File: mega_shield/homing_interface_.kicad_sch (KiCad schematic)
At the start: 15 parts, among them J8 T4040014031-000, J9 T4040014031-000, U14 4N35, U15 4N35

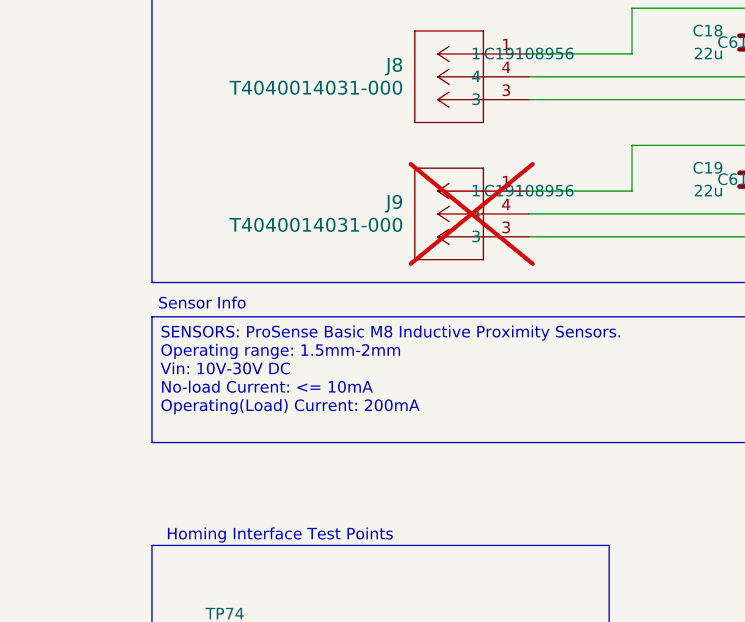
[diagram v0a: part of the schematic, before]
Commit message: replicated layout of homing interfaces. Placed the homing interface into PCB.
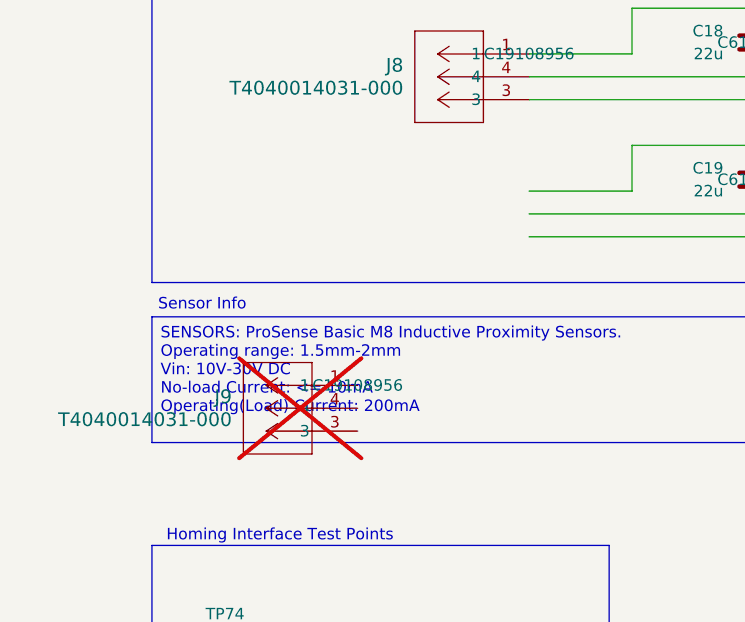
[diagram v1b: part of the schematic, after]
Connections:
- net +24V_IN: no longer J9.1
- net LIM_MAX_IN: no longer J9.3
- net at C19.2: no longer J9.4
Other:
- moved on the sheet: J9
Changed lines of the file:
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@@
 	(symbol
 		(lib_id "M8P3:T4040014031-000")
-		(at 67.31 62.23 0)
+		(at 48.26 83.82 0)
 		(mirror y)
 		(unit 1)
@@
 		(fields_autoplaced yes)
 		(property "Reference" "J9"
-			(at 53.34 63.4999 0)
+			(at 34.29 85.0899 0)
 			(effects
 				(font
@@
 		)
 		(property "Value" "T4040014031-000"
-			(at 53.34 66.0399 0)
+			(at 34.29 87.6299 0)
 			(effects
 				(font
@@
 		)
 		(property "Footprint" "footprints:CONN3_T4040014031-000_TEC"
-			(at 67.31 62.23 0)
+			(at 48.26 83.82 0)
 			(effects
 				(font
@@
 		)
 		(property "Datasheet" "T4040014031-000"
-			(at 67.31 62.23 0)
+			(at 48.26 83.82 0)
 			(effects
 				(font
@@
 		)
 		(property "Description" ""
-			(at 67.31 62.23 0)
+			(at 48.26 83.82 0)
 			(effects
 				(font
@@
 		)
 		(property "Purpose" ""
-			(at 67.31 62.23 0)
+			(at 48.26 83.82 0)
 			(effects
 				(font
@@
 		)
 		(property "jlcpcb" "C19108956"
-			(at 67.31 62.23 0)
+			(at 48.26 83.82 0)
 			(effects
 				(font

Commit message: fixed issue with shcematic connector having moved in homing interface sheet.
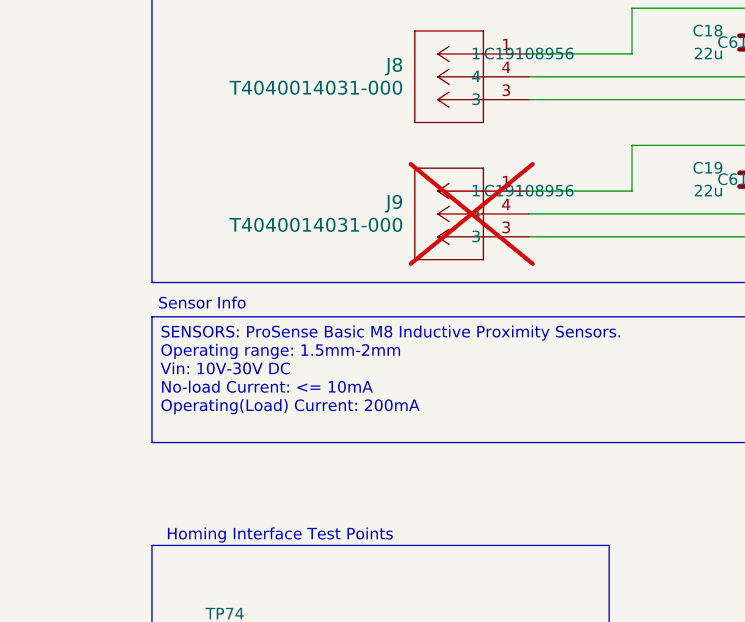
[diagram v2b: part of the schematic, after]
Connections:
- net +24V_IN: now also J9.1
- net LIM_MAX_IN: now also J9.3
- net at C19.2: now also J9.4
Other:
- moved on the sheet: J9
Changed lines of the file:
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@@
 	(symbol
 		(lib_id "M8P3:T4040014031-000")
-		(at 48.26 83.82 0)
+		(at 67.31 62.23 0)
 		(mirror y)
 		(unit 1)
@@
 		(fields_autoplaced yes)
 		(property "Reference" "J9"
-			(at 34.29 85.0899 0)
+			(at 53.34 63.4999 0)
 			(effects
 				(font
@@
 		)
 		(property "Value" "T4040014031-000"
-			(at 34.29 87.6299 0)
+			(at 53.34 66.0399 0)
 			(effects
 				(font
@@
 		)
 		(property "Footprint" "footprints:CONN3_T4040014031-000_TEC"
-			(at 48.26 83.82 0)
+			(at 67.31 62.23 0)
 			(effects
 				(font
@@
 		)
 		(property "Datasheet" "T4040014031-000"
-			(at 48.26 83.82 0)
+			(at 67.31 62.23 0)
 			(effects
 				(font
@@
 		)
 		(property "Description" ""
-			(at 48.26 83.82 0)
+			(at 67.31 62.23 0)
 			(effects
 				(font
@@
 		)
 		(property "Purpose" ""
-			(at 48.26 83.82 0)
+			(at 67.31 62.23 0)
 			(effects
 				(font
@@
 		)
 		(property "jlcpcb" "C19108956"
-			(at 48.26 83.82 0)
+			(at 67.31 62.23 0)
 			(effects
 				(font

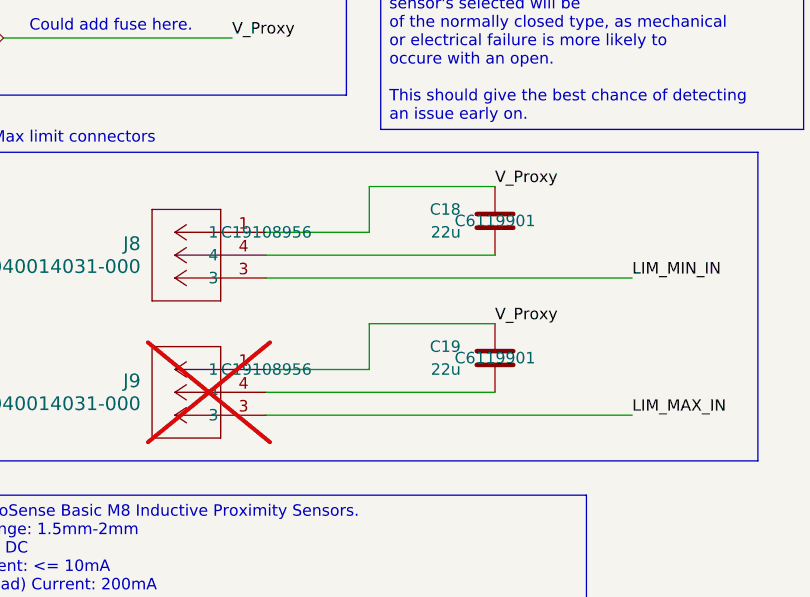
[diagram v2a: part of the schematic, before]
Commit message: mega_shield, Changed out all caps where needed for in-stock and lower cost parts.
+ Changed out for parts with higher stock.
+ Changed out for 0805 sized components.
+ Changed out for higher voltage.
+ Removed 22uF SMD caps for lower cost 10uF caps in parallel.
+ Updated diode footprint to SOD-123F

BOM cost reduced, and reliability improved.
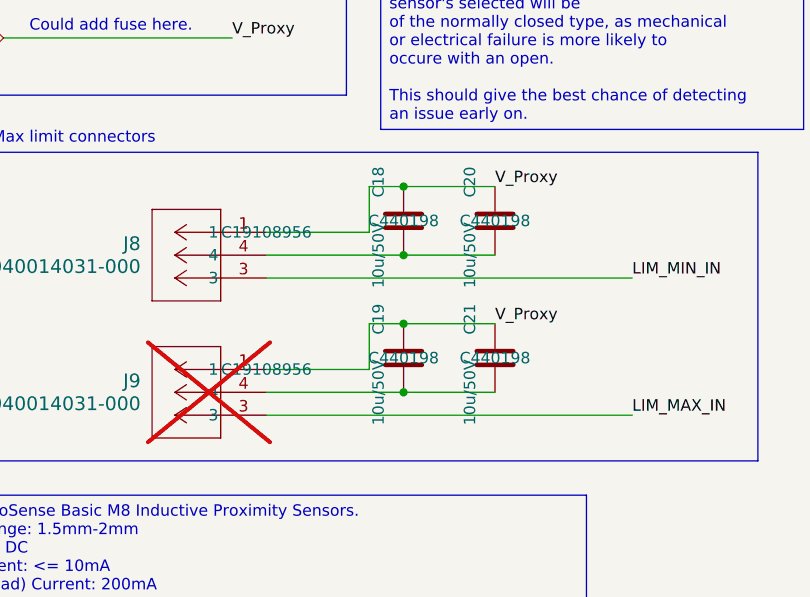
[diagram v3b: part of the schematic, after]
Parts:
- added C20, C21: 10u/50V, Capacitor_SMD:C_0805_2012Metric_Pad1.18x1.45mm_HandSolder, symbol Device:C
- C18, C19: value 22u -> 10u/50V; footprint Capacitor_SMD:C_0805_2012Metric -> Capacitor_SMD:C_0805_2012Metric_Pad1.18x1.45mm_HandSolder; jlcpcb C6119901 -> C440198
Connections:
- net +24V_IN: now also C20.1, C21.1
- net at C19.2, J9.4: now also C21.2
- net at C18.2, J8.4: now also C20.2
